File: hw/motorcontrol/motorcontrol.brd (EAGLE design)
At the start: 65 x 58 mm, 105 parts, among them J2 USB-MICROB, U1 BTN8982TA, U10 BSS138BKS, U11 DMG2305UX, U12 BSS138BKS, U2 BTN8982TA, U3 BTN8982TA, U4 CAT24C32WI-GT3, U5 ADG3304, U6 MMDT5401, U7 PTR08060W, U8 IPD90P03P4L-04, U9 ATMEGA32U4

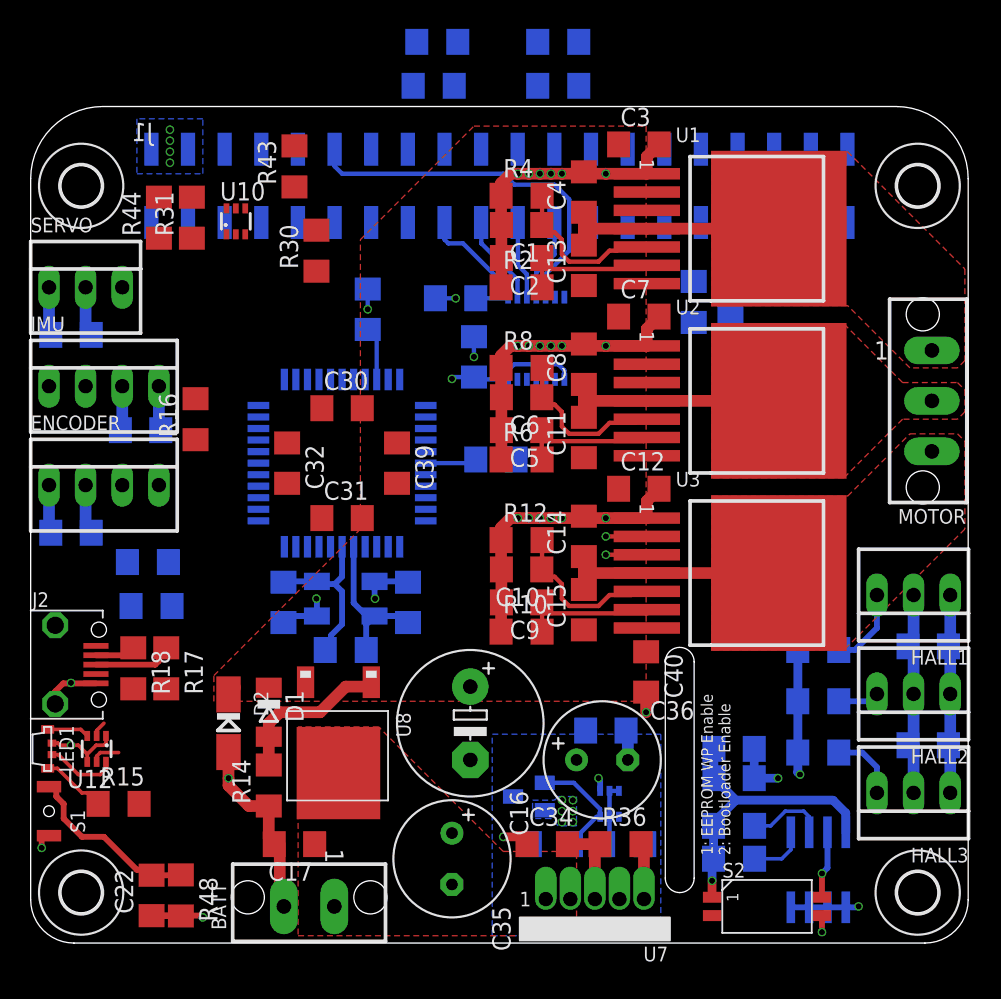
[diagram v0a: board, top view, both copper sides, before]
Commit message: backup
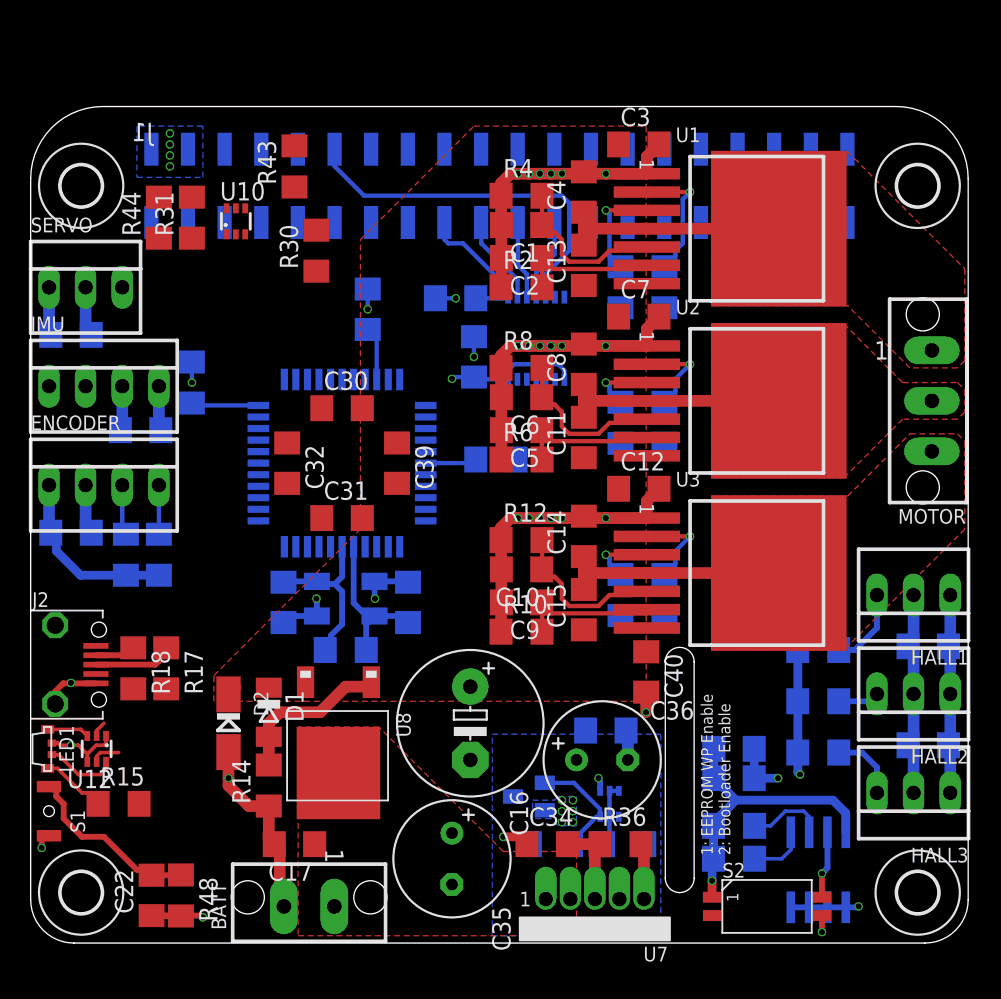
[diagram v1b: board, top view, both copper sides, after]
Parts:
- moved R9 38.6 mm to (40.9, 24.1), turned to 90 degrees
- moved R11 36.1 mm to (43.9, 24.1), turned to 90 degrees
- moved R7 30.8 mm to (43.9, 36.1), turned to 90 degrees
- moved R5 26.7 mm to (40.9, 36.1), turned to 90 degrees
- moved R1 5.18 mm to (40.9, 45.5)
- moved R3 4.60 mm to (43.9, 45.5)
- moved R27 3.59 mm to (8.89, 26.9), turned to 270 degrees
- moved R16 2.55 mm to (11.2, 38.9), flipped to the bottom
- moved R26 1.61 mm to (6.60, 26.9), turned to 270 degrees
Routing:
- net +5V: track 45.6 -> 56.2 mm, vias 14 -> 15
- net N$4: track 0.00 -> 8.92 mm, vias 0 -> 1
- net N$1: track 0.00 -> 7.17 mm, vias 0 -> 1
- net N$9: track 0.00 -> 6.38 mm, vias 0 -> 1
- net N$8: track 0.00 -> 4.68 mm
- net N$6: track 0.00 -> 4.63 mm, vias 0 -> 1
- net N$17: track 2.84 -> 6.38 mm
- net D4: track 0.00 -> 3.51 mm
- net D5: track 0.00 -> 3.40 mm
- net N$15: track 2.84 -> 4.63 mm
